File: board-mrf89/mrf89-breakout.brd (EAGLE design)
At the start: 100 x 80 mm, 21 parts, among them IC1 MRF89XA

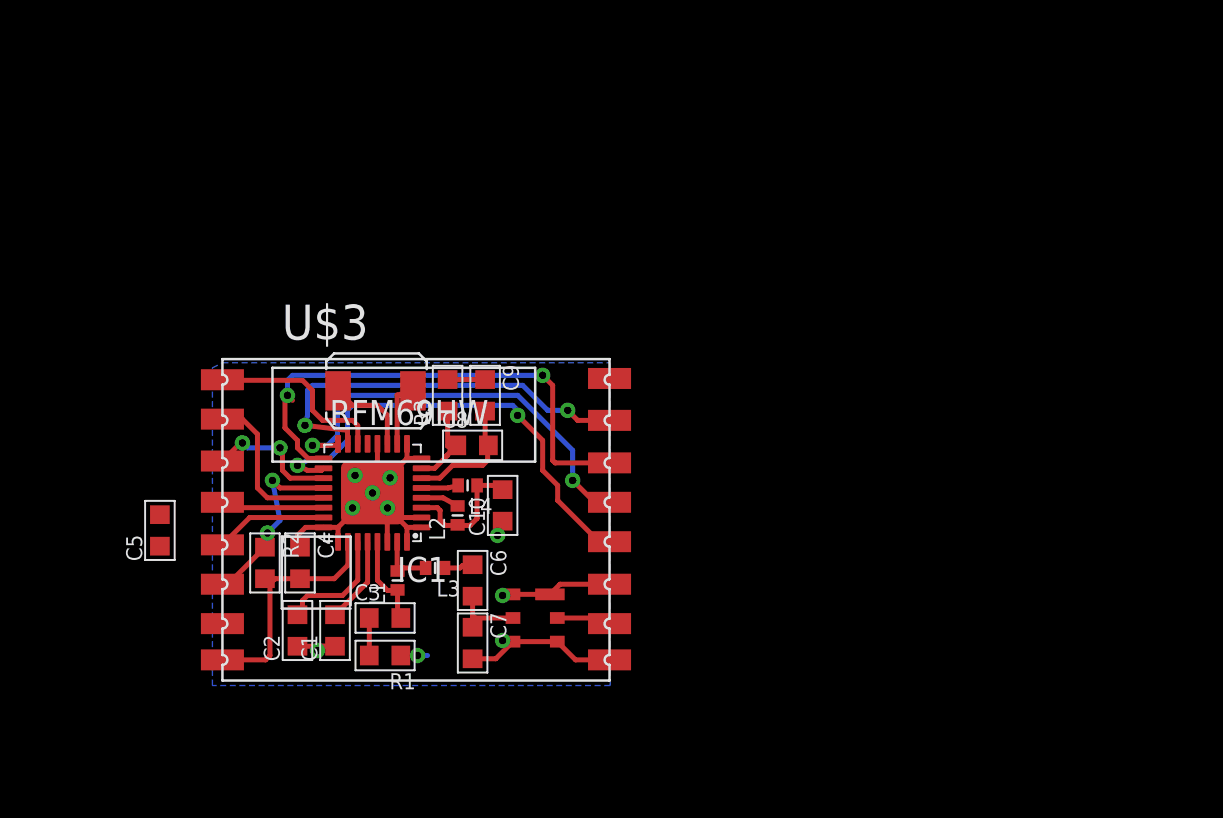
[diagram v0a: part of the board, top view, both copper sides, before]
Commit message: pretty much done
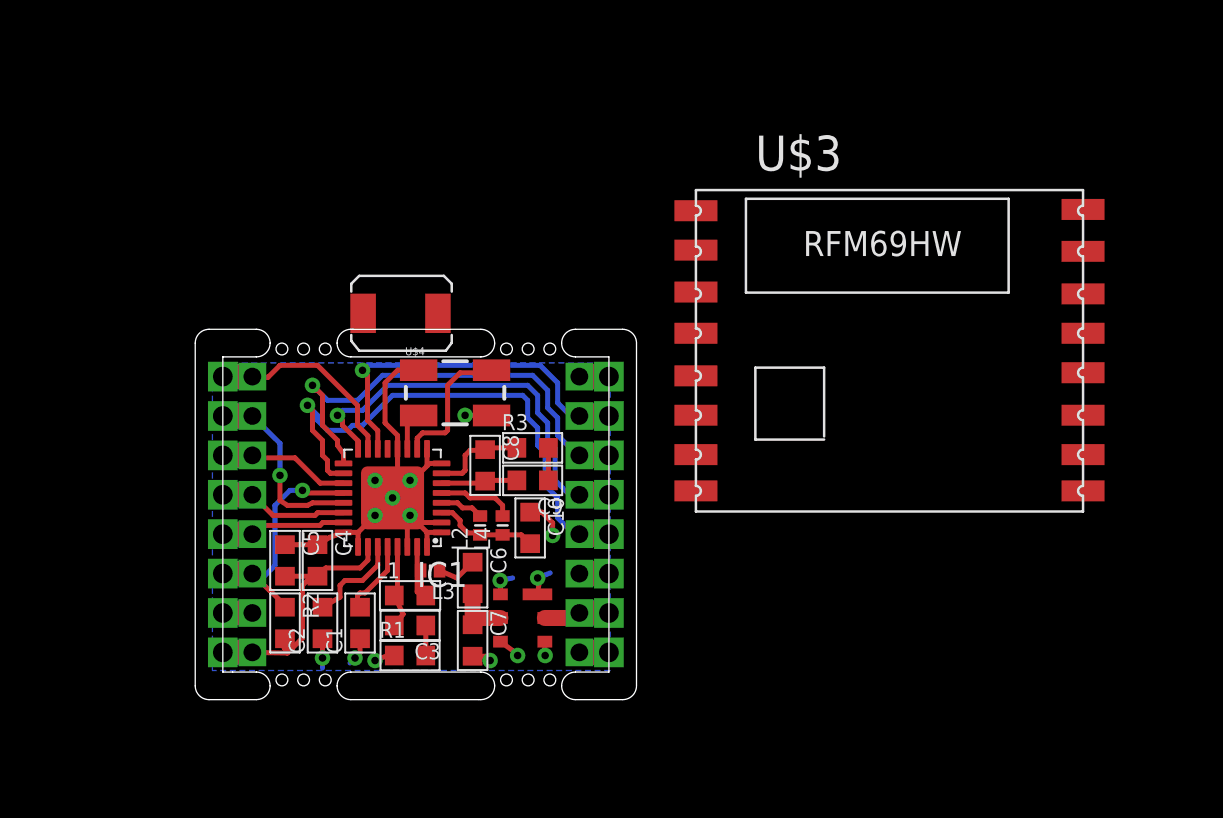
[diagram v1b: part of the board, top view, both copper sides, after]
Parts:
- added U$4: CRYSTAL-GROUNDED, SparkFun-FreqCtrl:CRYSTAL-SMD-5X3
- added U$5: BOARD-RADIO, Mine:BOARD-RADIO
- added U$6: (no value), Mine:BOARD-RADIO-CUTOUT
- C1: value (none) -> 220n
- C10: value (none) -> 100n
- C2, C4: value (none) -> 1u
- C3: value (none) -> 47n
- C5: value (none) -> 100p
- C8: value (none) -> 680p
- C9: value (none) -> 10n
- L1: value (none) -> 100n; device passives-7351:L0402-N -> passives-7351:L0603-N
- L2, L4: value (none) -> 6.8n
- R1: value (none) -> 1
- R2: value (none) -> 100k
- R3: value (none) -> 6.8k
- moved U$3 25.5 mm to (41.8, 22.6)
- moved C5 6.53 mm to (21.0, 20.1), turned to 270 degrees
- moved R3 5.08 mm to (33.5, 25.8), turned to 0 degrees
- moved C9 4.95 mm to (33.5, 24.1), turned to 180 degrees
- moved U$1 4.14 mm to (28.3, 32.5)
- moved R2 3.21 mm to (21.0, 16.9)
- moved L4 2.70 mm to (32.0, 21.8), turned to 90 degrees
- moved C10 1.81 mm to (33.4, 21.7), turned to 270 degrees
- moved C3 1.33 mm to (27.3, 16.8), turned to 180 degrees
- moved C1 1.33 mm to (24.8, 16.9)
- moved C2 1.33 mm to (22.9, 16.9)
- moved R1 1.27 mm to (27.3, 15.2), turned to 0 degrees
- moved L2 1.25 mm to (30.9, 21.8)
- moved C8 1.20 mm to (31.1, 24.9), turned to 270 degrees
- moved IC1 1.05 mm to (26.4, 23.2)
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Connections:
- removed net N$13: U$2.P$2, U$3.ANT
- removed net N$18: IC1.18, U$3.SCK
- removed net N$19: IC1.16, U$3.MISO
- removed net N$20: IC1.17, U$3.MOSI
- removed net N$21: IC1.15, U$3.NSS
- removed net N$22: IC1.14, U$3.RESET
- removed net N$23: IC1.21, U$3.DIO0
- new net ANT: U$2.P$2, U$5.10A, U$5.10B
- new net CSDAT: IC1.15, U$5.1A, U$5.1B
- new net IRQ0: IC1.21, U$5.2A, U$5.2B
- new net MISO: IC1.16, U$5.13A, U$5.13B
- new net MOSI: IC1.17, U$5.14A, U$5.14B
- new net N$38: U$5.16A, U$5.16B
- new net NSS: IC1.14, U$5.15A, U$5.15B
- new net SCK: IC1.18, U$5.12A, U$5.12B
- net +3V3: now also U$5.8A, U$5.8B; no longer U$3.VCC
- net DIO1: now also U$5.3A, U$5.3B; no longer U$3.DIO1
- net DIO2: now also U$5.4A, U$5.4B; no longer U$3.DIO2
- net DIO3: now also U$5.5A, U$5.5B; no longer U$3.DIO3
- net DIO4: now also U$5.6A, U$5.6B; no longer U$3.DIO4
- net DIO5: now also U$5.7A, U$5.7B; no longer U$3.DIO5
- net GND: now also U$4.2, U$4.4, U$5.11A, U$5.11B, U$5.9A, U$5.9B; no longer U$3.GNDA, U$3.GNDB
- net N$16: now also U$4.3
- net N$17: now also U$4.1
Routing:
- net N$20: track 26.2 -> 0.00 mm, vias 2 -> 0
- net SCK: track 0.00 -> 25.4 mm, vias 0 -> 1
- net N$18: track 23.7 -> 0.00 mm, vias 2 -> 0
- net MOSI: track 0.00 -> 21.9 mm, vias 0 -> 1
- net N$19: track 21.5 -> 0.00 mm, vias 2 -> 0
- net N$21: track 20.8 -> 0.00 mm, vias 2 -> 0
- net MISO: track 0.00 -> 19.4 mm, vias 0 -> 1
- net NSS: track 0.00 -> 17.1 mm, vias 0 -> 1
- net N$22: track 9.36 -> 0.00 mm
- net CSDAT: track 0.00 -> 8.86 mm
- net N$23: track 8.38 -> 0.00 mm
- net IRQ0: track 0.00 -> 8.20 mm, vias 0 -> 1
- net N$16: track 3.31 -> 7.06 mm
- net N$13: track 2.77 -> 0.00 mm
- net N$8: track 6.31 -> 3.84 mm
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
